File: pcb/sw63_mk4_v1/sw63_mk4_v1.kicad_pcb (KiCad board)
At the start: 4 copper layers, 35 x 35 mm, 70 parts, among them J1 GT-USB-7070C, J2 SWD, J3 Conn_01x02, Q1 DMG2305UX-7, Q2 DMG2302U-7, Q3 TEMT6200FX01, SW1 KSC321J LFS, SW2 ﻿EVQ-P7J01P, U1 DIO5518BST5, U2 MCP1711T-3.3I/OT, U3 TLC5916IPWR, U4 TLC5916IPWR, U5 TLC5916IPWR, U6 DS3231MZ, U7 STM32L052K8Ux

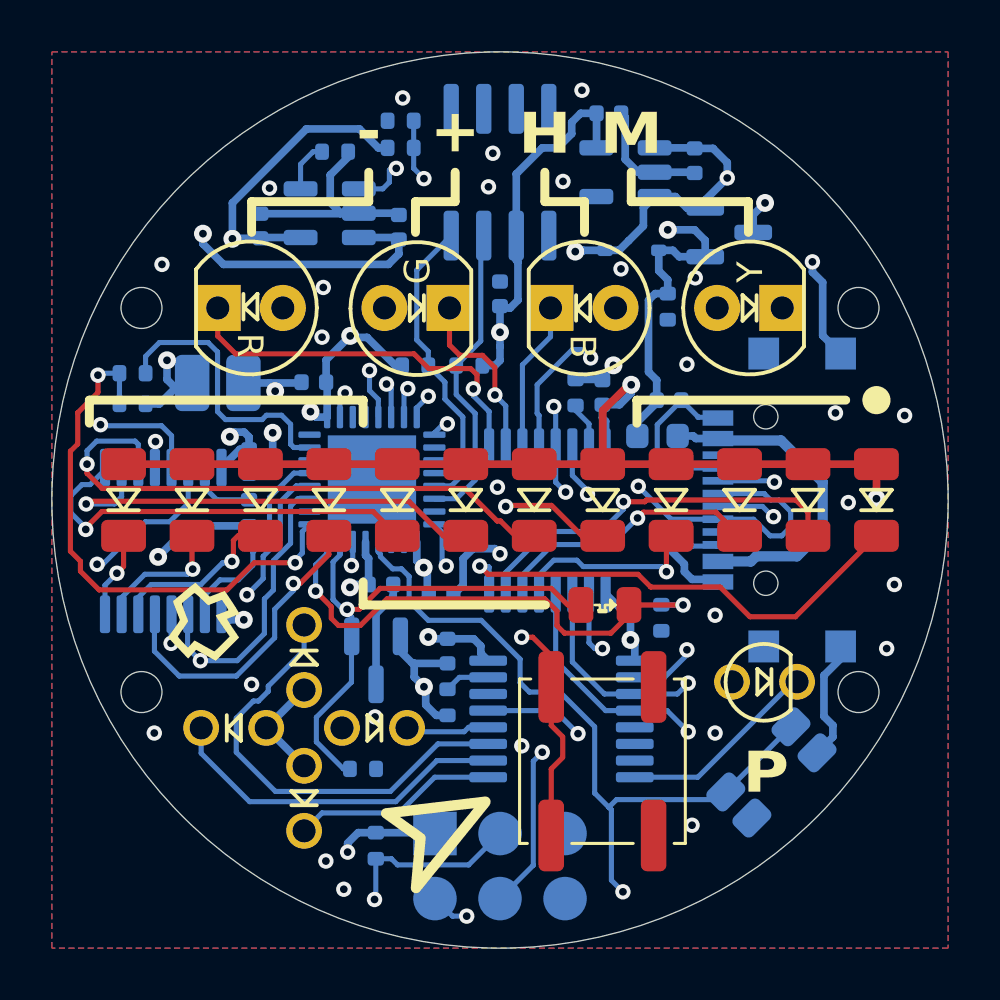
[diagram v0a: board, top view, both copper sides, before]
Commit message: update board
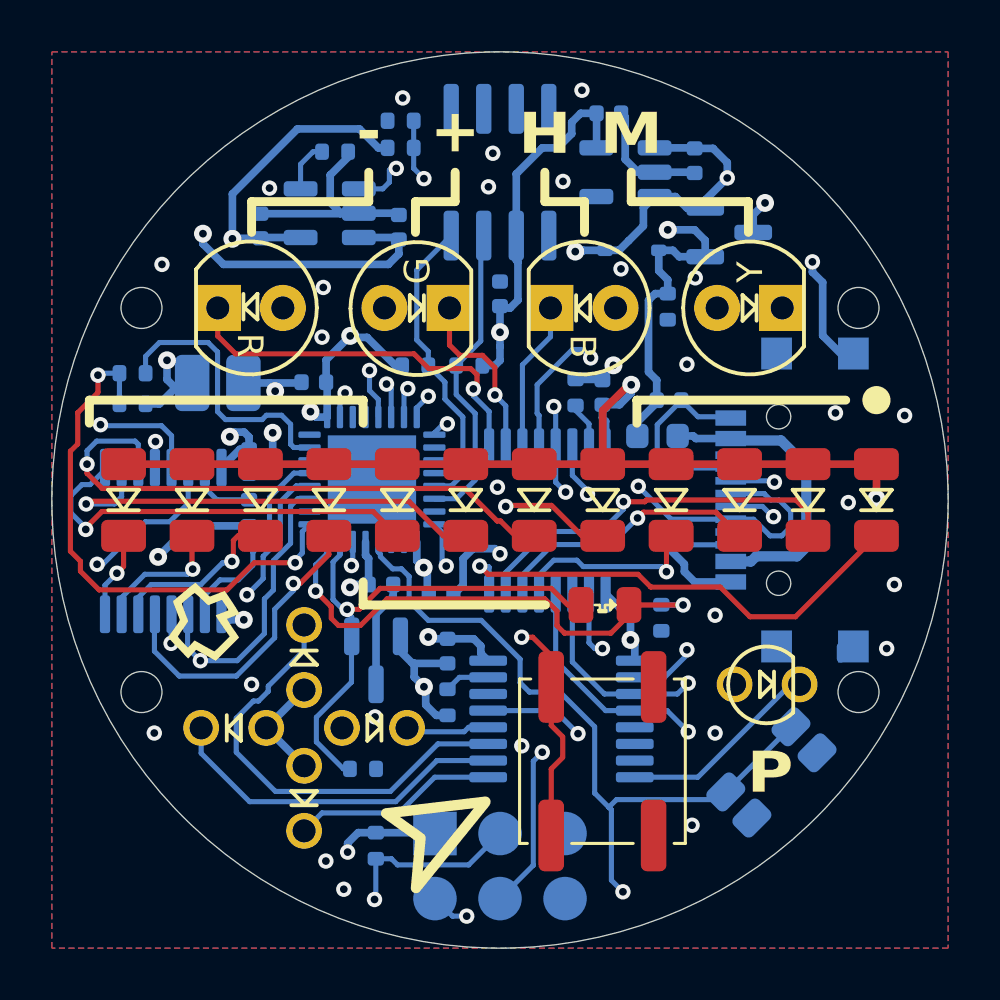
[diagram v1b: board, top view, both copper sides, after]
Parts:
- moved J1 0.50 mm to (131.3, 82.5)
- moved D21 0.14 mm to (129.2, 89.7)
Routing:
- net GND: track 40.3 -> 37.4 mm
- net Net-(F1-Pad1): track 13.0 -> 11.9 mm
- net /D-: track 26.6 -> 25.6 mm
- net Net-(J1-CC1): track 1.35 -> 1.85 mm
- net /D+: track 24.8 -> 24.3 mm
